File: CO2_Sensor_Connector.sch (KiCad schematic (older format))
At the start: 8 parts, among them J1 Conn_01x07_Female, J2 Conn_01x04_Female, Q1 AO3400A, Q2 AO3401A

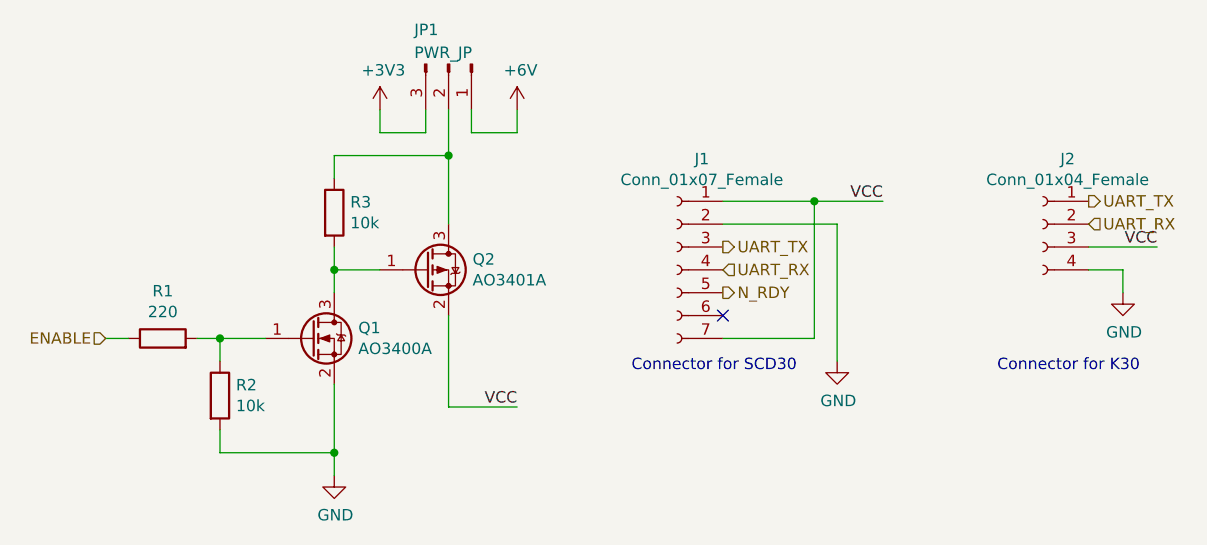
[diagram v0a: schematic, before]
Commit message: Start PCB layout
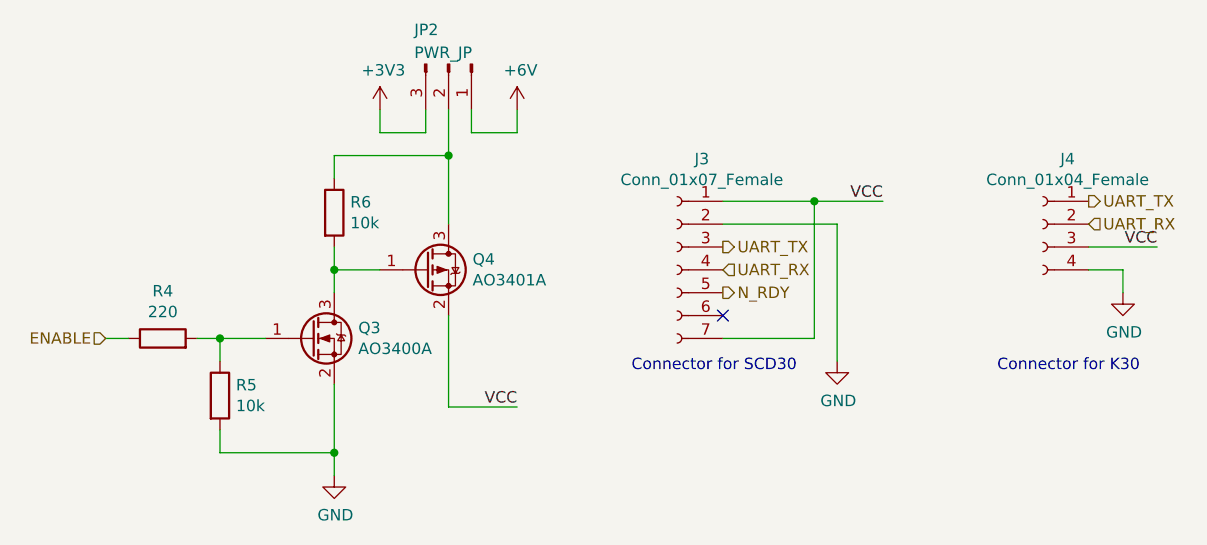
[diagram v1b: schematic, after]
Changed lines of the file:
@@
 AR Path="/60A49A7C/60A57B40" Ref="J1"  Part="1"
 AR Path="/60A4AC4A/60A57B40" Ref="J3"  Part="1"
-F 0 "J1" H 5692 4385 50  0000 C CNN
+F 0 "J3" H 5692 4385 50  0000 C CNN
 F 1 "Conn_01x07_Female" H 5692 4294 50  0000 C CNN
 F 2 "Connector_PinSocket_2.54mm:PinSocket_1x07_P2.54mm_Vertical" H 5800 3900 50  0001 C CNN
@@
 AR Path="/60A49A7C/60A6C14D" Ref="Q2"  Part="1"
 AR Path="/60A4AC4A/60A6C14D" Ref="Q4"  Part="1"
-F 0 "Q2" H 4905 3946 50  0000 L CNN
+F 0 "Q4" H 4905 3946 50  0000 L CNN
 F 1 "AO3401A" H 4905 3855 50  0000 L CNN
 F 2 "Package_TO_SOT_SMD:SOT-23" H 4900 3825 50  0001 L CIN
@@
 AR Path="/60A49A7C/60A6FA21" Ref="R1"  Part="1"
 AR Path="/60A4AC4A/60A6FA21" Ref="R4"  Part="1"
-F 0 "R1" V 3757 4200 50  0000 C CNN
+F 0 "R4" V 3757 4200 50  0000 C CNN
 F 1 "220" V 3666 4200 50  0000 C CNN
 F 2 "Resistor_SMD:R_0603_1608Metric" V 3480 4200 50  0001 C CNN
@@
 AR Path="/60A49A7C/60A736D3" Ref="R3"  Part="1"
 AR Path="/60A4AC4A/60A736D3" Ref="R6"  Part="1"
-F 0 "R3" H 4370 3696 50  0000 L CNN
+F 0 "R6" H 4370 3696 50  0000 L CNN
 F 1 "10k" H 4370 3605 50  0000 L CNN
 F 2 "Resistor_SMD:R_0603_1608Metric" V 4230 3650 50  0001 C CNN
@@
 AR Path="/60A49A7C/60A91C0B" Ref="JP1"  Part="1"
 AR Path="/60A4AC4A/60A91C0B" Ref="JP2"  Part="1"
-F 0 "JP1" V 4650 2850 50  0000 L CNN
+F 0 "JP2" V 4650 2850 50  0000 L CNN
 F 1 "PWR_JP" V 4750 2850 50  0000 L CNN
 F 2 "Connector_PinHeader_2.54mm:PinHeader_1x03_P2.54mm_Vertical" H 4800 3000 50  0001 C CNN
@@
 AR Path="/60A49A7C/60AA508F" Ref="R2"  Part="1"
 AR Path="/60A4AC4A/60AA508F" Ref="R5"  Part="1"
-F 0 "R2" H 3870 4496 50  0000 L CNN
+F 0 "R5" H 3870 4496 50  0000 L CNN
 F 1 "10k" H 3870 4405 50  0000 L CNN
 F 2 "Resistor_SMD:R_0603_1608Metric" V 3730 4450 50  0001 C CNN
@@
 AR Path="/60A49A7C/60ABE2B1" Ref="J2"  Part="1"
 AR Path="/60A4AC4A/60ABE2B1" Ref="J4"  Part="1"
-F 0 "J2" H 7292 3985 50  0000 C CNN
+F 0 "J4" H 7292 3985 50  0000 C CNN
 F 1 "Conn_01x04_Female" H 7292 3894 50  0000 C CNN
 F 2 "Connector_PinSocket_2.54mm:PinSocket_1x04_P2.54mm_Vertical" H 7400 3700 50  0001 C CNN
@@
 AR Path="/60A49A7C/60B57C20" Ref="Q1"  Part="1"
 AR Path="/60A4AC4A/60B57C20" Ref="Q3"  Part="1"
-F 0 "Q1" H 4405 4246 50  0000 L CNN
+F 0 "Q3" H 4405 4246 50  0000 L CNN
 F 1 "AO3400A" H 4405 4155 50  0000 L CNN
 F 2 "Package_TO_SOT_SMD:SOT-23" H 4400 4125 50  0001 L CIN

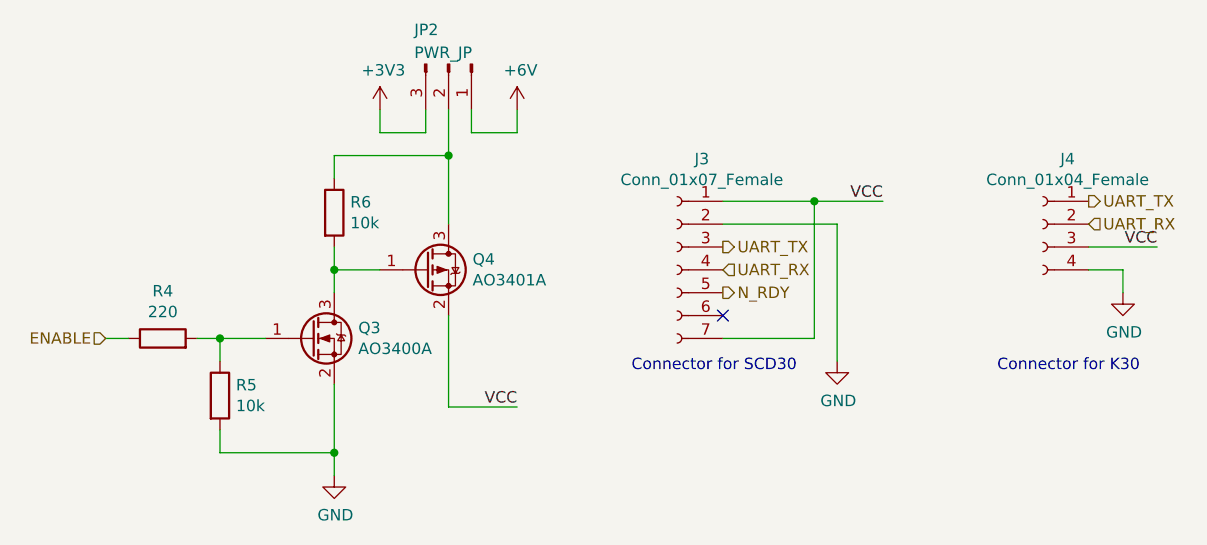
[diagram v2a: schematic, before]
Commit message: Layout complete, barring review and polish
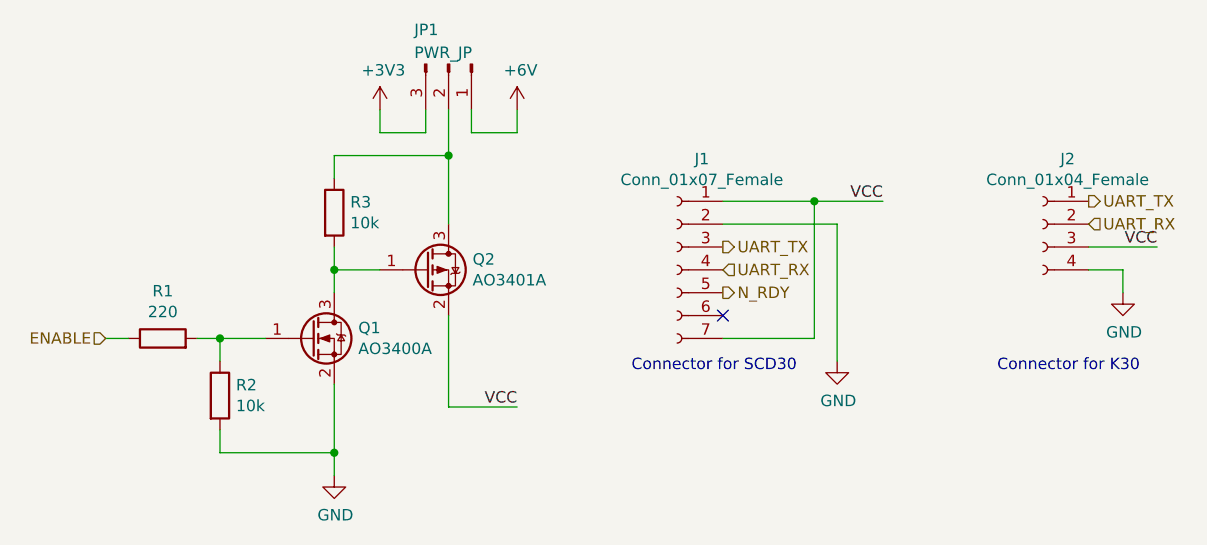
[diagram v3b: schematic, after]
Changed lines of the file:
@@
 $Descr A4 11693 8268
 encoding utf-8
-Sheet 3 9
+Sheet 2 9
 Title ""
 Date ""
@@
 AR Path="/60A49A7C/60A57B40" Ref="J1"  Part="1"
 AR Path="/60A4AC4A/60A57B40" Ref="J3"  Part="1"
-F 0 "J3" H 5692 4385 50  0000 C CNN
+F 0 "J1" H 5692 4385 50  0000 C CNN
 F 1 "Conn_01x07_Female" H 5692 4294 50  0000 C CNN
 F 2 "Connector_PinSocket_2.54mm:PinSocket_1x07_P2.54mm_Vertical" H 5800 3900 50  0001 C CNN
@@
 AR Path="/60A49A7C/60A5D6A7" Ref="#PWR04"  Part="1"
 AR Path="/60A4AC4A/60A5D6A7" Ref="#PWR09"  Part="1"
-F 0 "#PWR09" H 6500 4050 50  0001 C CNN
+F 0 "#PWR04" H 6500 4050 50  0001 C CNN
 F 1 "GND" H 6505 4127 50  0000 C CNN
 F 2 "" H 6500 4300 50  0001 C CNN
@@
 AR Path="/60A49A7C/60A6C14D" Ref="Q2"  Part="1"
 AR Path="/60A4AC4A/60A6C14D" Ref="Q4"  Part="1"
-F 0 "Q4" H 4905 3946 50  0000 L CNN
+F 0 "Q2" H 4905 3946 50  0000 L CNN
 F 1 "AO3401A" H 4905 3855 50  0000 L CNN
 F 2 "Package_TO_SOT_SMD:SOT-23" H 4900 3825 50  0001 L CIN
@@
 AR Path="/60A49A7C/60A6FA21" Ref="R1"  Part="1"
 AR Path="/60A4AC4A/60A6FA21" Ref="R4"  Part="1"
-F 0 "R4" V 3757 4200 50  0000 C CNN
+F 0 "R1" V 3757 4200 50  0000 C CNN
 F 1 "220" V 3666 4200 50  0000 C CNN
 F 2 "Resistor_SMD:R_0603_1608Metric" V 3480 4200 50  0001 C CNN
@@
 AR Path="/60A49A7C/60A736D3" Ref="R3"  Part="1"
 AR Path="/60A4AC4A/60A736D3" Ref="R6"  Part="1"
-F 0 "R6" H 4370 3696 50  0000 L CNN
+F 0 "R3" H 4370 3696 50  0000 L CNN
 F 1 "10k" H 4370 3605 50  0000 L CNN
 F 2 "Resistor_SMD:R_0603_1608Metric" V 4230 3650 50  0001 C CNN
@@
 AR Path="/60A49A7C/60A91C0B" Ref="JP1"  Part="1"
 AR Path="/60A4AC4A/60A91C0B" Ref="JP2"  Part="1"
-F 0 "JP2" V 4650 2850 50  0000 L CNN
+F 0 "JP1" V 4650 2850 50  0000 L CNN
 F 1 "PWR_JP" V 4750 2850 50  0000 L CNN
 F 2 "Connector_PinHeader_2.54mm:PinHeader_1x03_P2.54mm_Vertical" H 4800 3000 50  0001 C CNN
@@
 AR Path="/60A49A7C/60A94D4D" Ref="#PWR02"  Part="1"
 AR Path="/60A4AC4A/60A94D4D" Ref="#PWR07"  Part="1"
-F 0 "#PWR07" H 4500 3050 50  0001 C CNN
+F 0 "#PWR02" H 4500 3050 50  0001 C CNN
 F 1 "+3V3" H 4515 3373 50  0000 C CNN
 F 2 "" H 4500 3200 50  0001 C CNN
@@
 AR Path="/60A49A7C/60A9539A" Ref="#PWR03"  Part="1"
 AR Path="/60A4AC4A/60A9539A" Ref="#PWR08"  Part="1"
-F 0 "#PWR08" H 5100 3050 50  0001 C CNN
+F 0 "#PWR03" H 5100 3050 50  0001 C CNN
 F 1 "+6V" H 5115 3373 50  0000 C CNN
 F 2 "" H 5100 3200 50  0001 C CNN
@@
 AR Path="/60A49A7C/60A9EA13" Ref="#PWR01"  Part="1"
 AR Path="/60A4AC4A/60A9EA13" Ref="#PWR06"  Part="1"
-F 0 "#PWR06" H 4300 4550 50  0001 C CNN
+F 0 "#PWR01" H 4300 4550 50  0001 C CNN
 F 1 "GND" H 4305 4627 50  0000 C CNN
 F 2 "" H 4300 4800 50  0001 C CNN
@@
 AR Path="/60A49A7C/60AA508F" Ref="R2"  Part="1"
 AR Path="/60A4AC4A/60AA508F" Ref="R5"  Part="1"
-F 0 "R5" H 3870 4496 50  0000 L CNN
+F 0 "R2" H 3870 4496 50  0000 L CNN
 F 1 "10k" H 3870 4405 50  0000 L CNN
 F 2 "Resistor_SMD:R_0603_1608Metric" V 3730 4450 50  0001 C CNN
@@
 AR Path="/60A49A7C/60ABDE86" Ref="#PWR05"  Part="1"
 AR Path="/60A4AC4A/60ABDE86" Ref="#PWR010"  Part="1"
-F 0 "#PWR010" H 7750 3750 50  0001 C CNN
+F 0 "#PWR05" H 7750 3750 50  0001 C CNN
 F 1 "GND" H 7755 3827 50  0000 C CNN
 F 2 "" H 7750 4000 50  0001 C CNN
@@
 AR Path="/60A49A7C/60ABE2B1" Ref="J2"  Part="1"
 AR Path="/60A4AC4A/60ABE2B1" Ref="J4"  Part="1"
-F 0 "J4" H 7292 3985 50  0000 C CNN
+F 0 "J2" H 7292 3985 50  0000 C CNN
 F 1 "Conn_01x04_Female" H 7292 3894 50  0000 C CNN
 F 2 "Connector_PinSocket_2.54mm:PinSocket_1x04_P2.54mm_Vertical" H 7400 3700 50  0001 C CNN
@@
 AR Path="/60A49A7C/60B57C20" Ref="Q1"  Part="1"
 AR Path="/60A4AC4A/60B57C20" Ref="Q3"  Part="1"
-F 0 "Q3" H 4405 4246 50  0000 L CNN
+F 0 "Q1" H 4405 4246 50  0000 L CNN
 F 1 "AO3400A" H 4405 4155 50  0000 L CNN
 F 2 "Package_TO_SOT_SMD:SOT-23" H 4400 4125 50  0001 L CIN
